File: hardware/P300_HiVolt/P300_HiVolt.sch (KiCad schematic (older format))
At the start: 10 parts, among them J1 Conn_01x02, J2 Conn_01x08, J3 Stiftleiste 6P - Molex, J4 Stiftleiste 6P - Molex, J5 12V, J6 5V, T1 HLK-PM12, T2 HLK-PM05

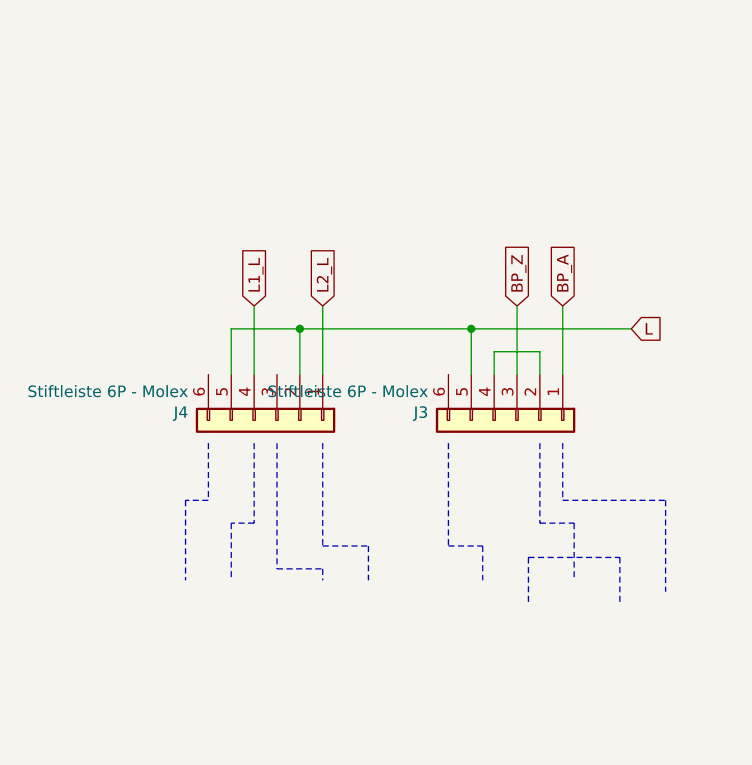
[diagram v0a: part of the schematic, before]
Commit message: Platinen V.23 in die Herstellung gegeben
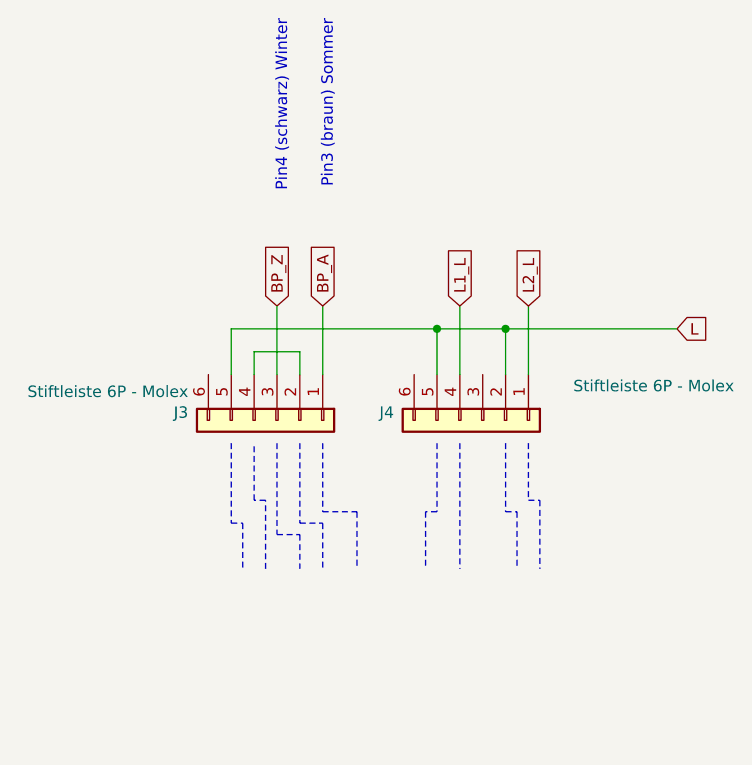
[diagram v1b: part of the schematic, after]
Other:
- note added: "Pin3 (braun) Sommer"
- note added: "Pin4 (schwarz) Winter"
- moved on the sheet: J3, J4
